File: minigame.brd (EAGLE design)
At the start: 98.7 x 80 mm, 44 parts, among them J1 AVR_SPI_PRG_6PTH, Q1 MMBT2222A, U1 MCP73831, U2 MIC5219 3.3V, Y1 8MHz

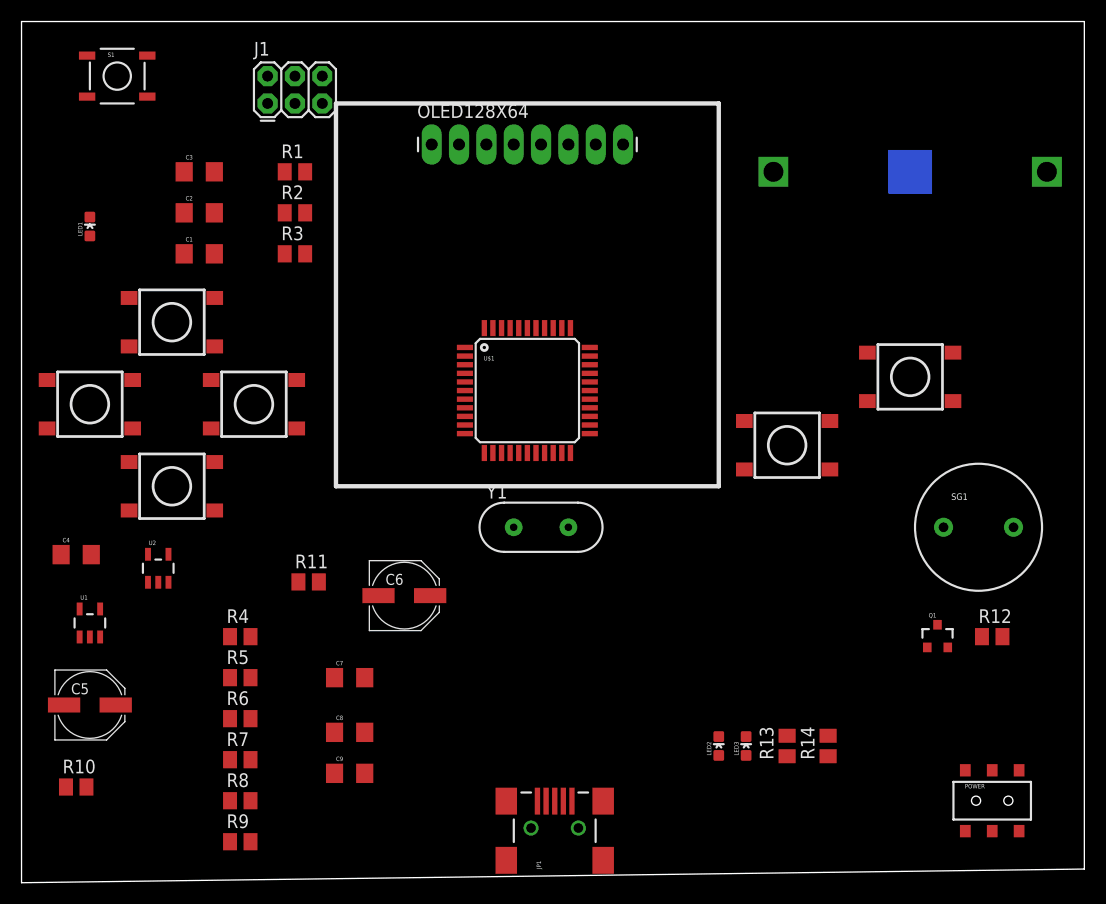
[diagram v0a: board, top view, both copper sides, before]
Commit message: Preliminary components placement
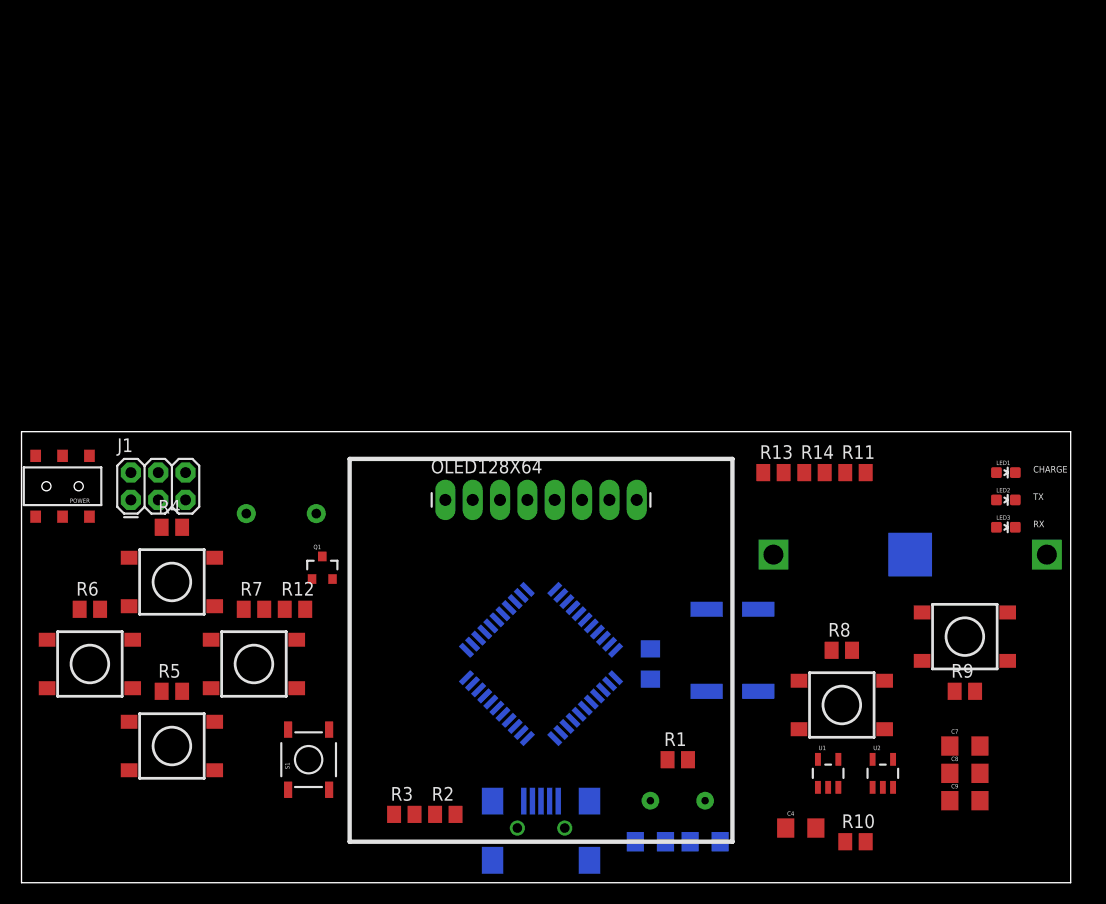
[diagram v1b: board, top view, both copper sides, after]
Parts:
- moved POWER 91.2 mm to (3.81, 36.8), turned to 180 degrees
- moved LED1 88.1 mm to (91.4, 38.1), turned to 270 degrees
- moved R10 72.6 mm to (77.5, 3.81)
- moved C1 72.0 mm to (63.5, 3.81), flipped to the bottom
- moved C4 71.9 mm to (72.4, 5.08)
- moved C2 71.9 mm to (58.4, 3.81), flipped to the bottom
- moved U1 70.0 mm to (74.9, 10.2)
- moved U2 70.0 mm to (80.0, 10.2)
- moved R9 68.7 mm to (87.6, 17.8)
- moved S1 65.9 mm to (26.7, 11.4), turned to 90 degrees
- moved R1 65.2 mm to (61.0, 11.4)
- moved R12 64.8 mm to (25.4, 25.4)
- moved SG1 64.8 mm to (24.1, 34.3), flipped to the bottom
- moved C3 62.0 mm to (58.4, 20.3), flipped to the bottom, turned to 90 degrees
- moved C5 60.3 mm to (66.0, 25.4), flipped to the bottom
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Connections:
- removed net OLED_3V3: OLED128X64.6
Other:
- board size 98.7 x 80 mm -> 97.5 x 41.9 mm
- board text added: "CHARGE"
- board text added: "RX"
- board text added: "TX"
